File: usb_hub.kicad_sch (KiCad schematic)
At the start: 15 parts, among them U2 USB2514B_Bi, Y1 ABLS-24.000MHZ-B4-T

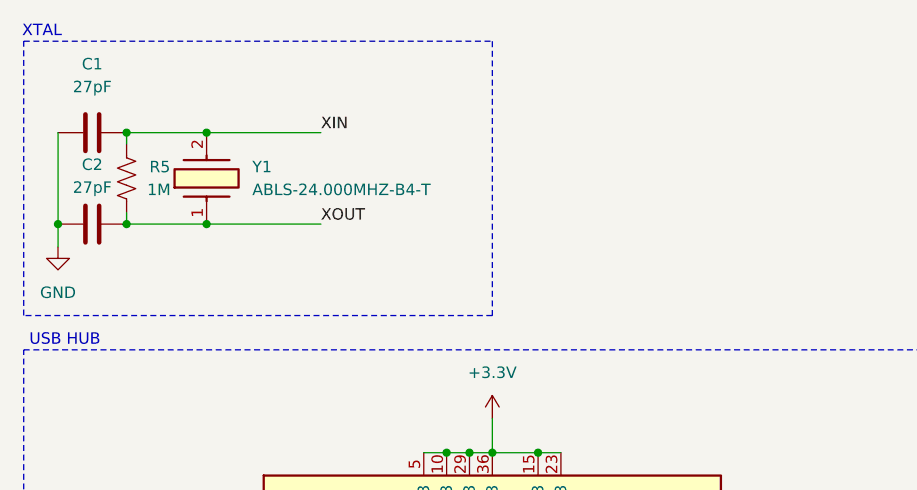
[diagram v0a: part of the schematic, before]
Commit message: routed stm32
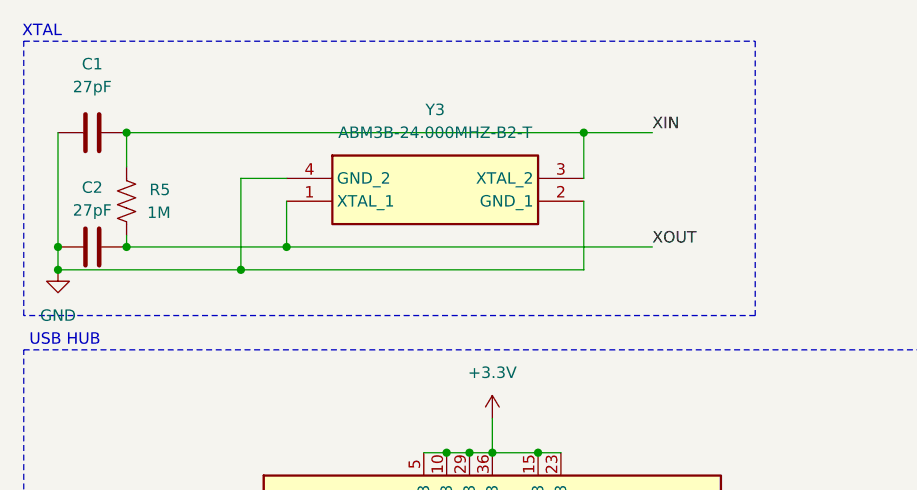
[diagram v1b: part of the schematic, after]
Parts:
- removed Y1: ABLS-24.000MHZ-B4-T, ABLS24000MHZB4T, symbol SamacSys_Parts:ABLS-24.000MHZ-B4-T
- added Y3: ABM3B-24.000MHZ-B2-T, ABM3B, symbol SamacSys_Parts:ABM3B-24.000MHZ-B2-T
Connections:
- net GND: now also Y3.2 (GND_1), Y3.4 (GND_2)
- net XIN: now also Y3.3 (XTAL_2)
- net XOUT: now also Y3.1 (XTAL_1)
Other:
- moved on the sheet: C2, R5
